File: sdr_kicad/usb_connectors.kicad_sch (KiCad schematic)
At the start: 10 parts, among them J1 USB_C_Receptacle, J2 USB_C_Receptacle, U10 USBLC6-2SC6, U11 USBLC6-2SC6

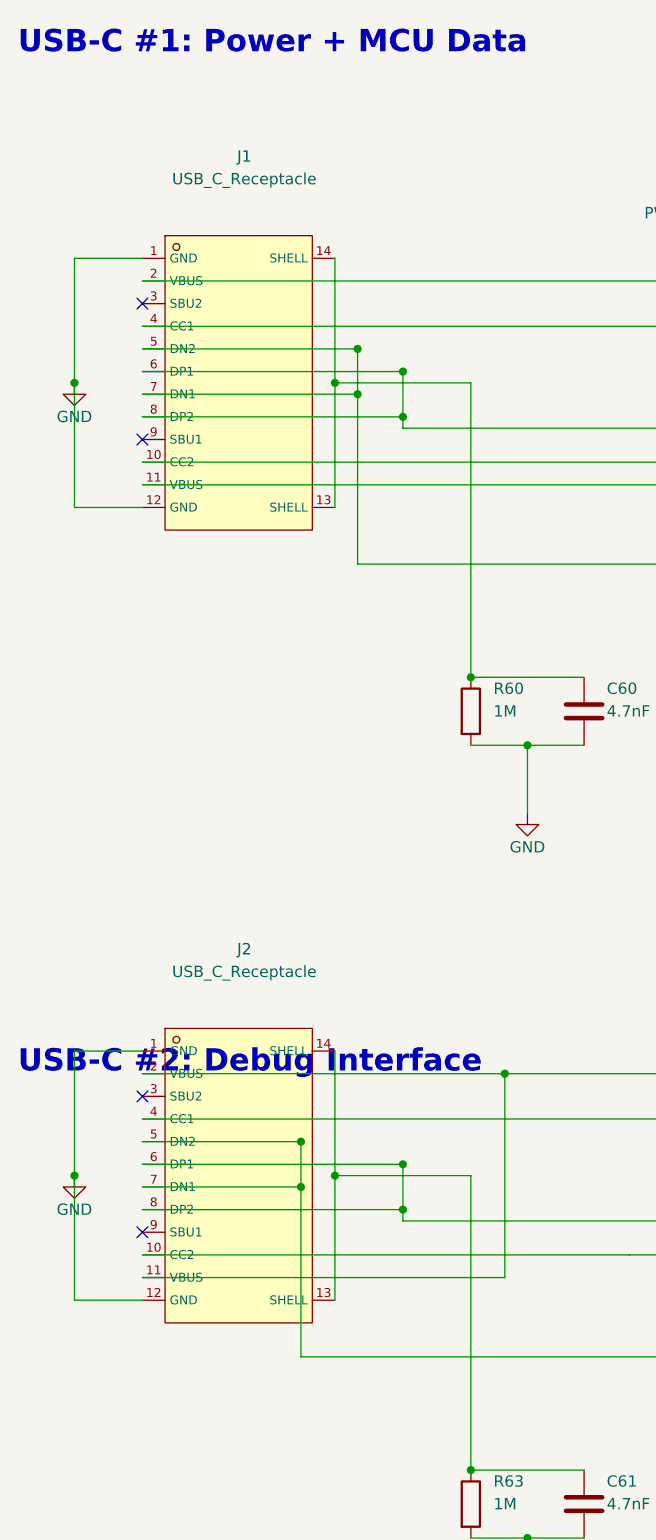
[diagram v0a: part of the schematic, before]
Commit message: add firmware and readme
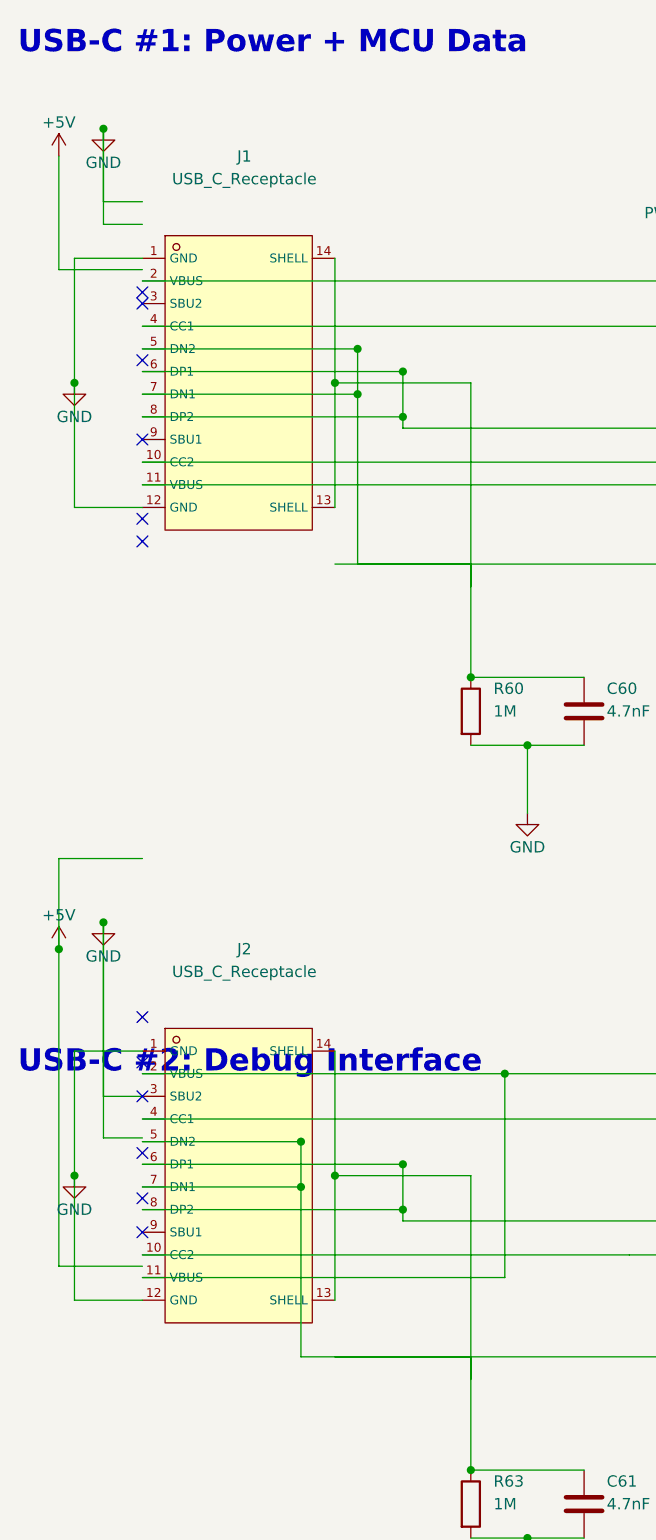
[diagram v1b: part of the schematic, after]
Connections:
- net GND: now also C61.1, J2.13 (SHELL), J2.14 (SHELL), J2.3 (SBU2), R63.1
- net at C60.1, J1.13 (SHELL), J1.14 (SHELL)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: now also J1.5 (DN2), J1.7 (DN1), U10.3 (I/O2)
- no-connect marks 4 -> 12
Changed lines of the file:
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@@
   (junction (at 76.2 96.52) (diameter 0) (color 0 0 0 0) (uuid "jct-rc1-top"))
   (junction (at 76.2 185.42) (diameter 0) (color 0 0 0 0) (uuid "jct-rc2-top"))
+  ; J1 missing connections
+  ; GND pins
+  (wire (pts (xy 39.37 45.72) (xy 35 45.72)) (uuid "wire-j1-gnd1-1"))
+  (wire (pts (xy 35 45.72) (xy 35 35)) (uuid "wire-j1-gnd1-2"))
+  (wire (pts (xy 39.37 43.18) (xy 35 43.18)) (uuid "wire-j1-gnd12-1"))
+  (wire (pts (xy 35 43.18) (xy 35 35)) (uuid "wire-j1-gnd12-2"))
+  (junction (at 35 35) (uuid "jct-j1-gnd"))
+  (symbol
+    (lib_id "power:GND")
+    (at 35 35 0)
+    (unit 1)
+    (exclude_from_sim no)
+    (in_bom no)
+    (on_board yes)
+    (dnp no)
+    (uuid "pwr-gnd-j1")
+    (property "Reference" "#PWR017"
+      (at 35 41.35 0)
+      (effects (font (size 1.27 1.27)) hide)
+    )
+    (property "Value" "GND"
+      (at 35 38.81 0)
+      (effects (font (size 1.27 1.27)))
+    )
+  )
+  ; VBUS pin 11
+  (wire (pts (xy 39.37 50.80) (xy 30 50.80)) (uuid "wire-j1-vbus11-1"))
+  (wire (pts (xy 30 50.80) (xy 30 38.1)) (uuid "wire-j1-vbus11-2"))
+  (symbol
+    (lib_id "power:+5V")
+    (at 30 38.1 0)
+    (unit 1)
+    (exclude_from_sim no)
+    (in_bom no)
+    (on_board yes)
+    (dnp no)
+    (uuid "pwr-5v-j1-vbus11")
+    (property "Reference" "#PWR018"
+      (at 30 41.91 0)
+      (effects (font (size 1.27 1.27)) hide)
+    )
+    (property "Value" "+5V"
+      (at 30 34.29 0)
+      (effects (font (size 1.27 1.27)))
+    )
+  )
+  ; SHELL pin 13
+  (wire (pts (xy 60.96 83.82) (xy 76.2 83.82)) (uuid "wire-j1-shell13-1"))
+  (wire (pts (xy 76.2 83.82) (xy 76.2 86.36)) (uuid "wire-j1-shell13-2"))
+  ; No-connect flags for J1
+  (no_connect (at 39.37 53.34) (uuid "nc-j1-sbu2"))
+  (no_connect (at 39.37 60.96) (uuid "nc-j1-dn2"))
+  (no_connect (at 39.37 78.74) (uuid "nc-j1-dp2"))
+  (no_connect (at 39.37 81.28) (uuid "nc-j1-sbu1"))
+  ; J2 missing connections
+  ; GND pins
+  (wire (pts (xy 39.37 143.51) (xy 35 143.51)) (uuid "wire-j2-gnd1-1"))
+  (wire (pts (xy 35 143.51) (xy 35 124)) (uuid "wire-j2-gnd1-2"))
+  (wire (pts (xy 39.37 148.17) (xy 35 148.17)) (uuid "wire-j2-gnd12-1"))
+  (wire (pts (xy 35 148.17) (xy 35 124)) (uuid "wire-j2-gnd12-2"))
+  (junction (at 35 124) (uuid "jct-j2-gnd"))
+  (symbol
+    (lib_id "power:GND")
+    (at 35 124 0)
+    (unit 1)
+    (exclude_from_sim no)
+    (in_bom no)
+    (on_board yes)
+    (dnp no)
+    (uuid "pwr-gnd-j2")
+    (property "Reference" "#PWR019"
+      (at 35 130.35 0)
+      (effects (font (size 1.27 1.27)) hide)
+    )
+    (property "Value" "GND"
+      (at 35 127.81 0)
+      (effects (font (size 1.27 1.27)))
+    )
+  )
+  ; VBUS pins 2 and 11
+  (wire (pts (xy 39.37 116.84) (xy 30 116.84)) (uuid "wire-j2-vbus2-1"))
+  (wire (pts (xy 30 116.84) (xy 30 127)) (uuid "wire-j2-vbus2-2"))
+  (wire (pts (xy 39.37 162.56) (xy 30 162.56)) (uuid "wire-j2-vbus11-1"))
+  (wire (pts (xy 30 162.56) (xy 30 127)) (uuid "wire-j2-vbus11-2"))
+  (junction (at 30 127) (uuid "jct-j2-vbus"))
+  (symbol
+    (lib_id "power:+5V")
+    (at 30 127 0)
+    (unit 1)
+    (exclude_from_sim no)
+    (in_bom no)
+    (on_board yes)
+    (dnp no)
+    (uuid "pwr-5v-j2-vbus")
+    (property "Reference" "#PWR020"
+      (at 30 130.81 0)
+      (effects (font (size 1.27 1.27)) hide)
+    )
+    (property "Value" "+5V"
+      (at 30 123.19 0)
+      (effects (font (size 1.27 1.27)))
+    )
+  )
+  ; SHELL pin 13
+  (wire (pts (xy 60.96 172.72) (xy 76.2 172.72)) (uuid "wire-j2-shell13-1"))
+  (wire (pts (xy 76.2 172.72) (xy 76.2 175.26)) (uuid "wire-j2-shell13-2"))
+  ; No-connect flags for J2
+  (no_connect (at 39.37 134.62) (uuid "nc-j2-sbu2"))
+  (no_connect (at 39.37 139.7) (uuid "nc-j2-dn2"))
+  (no_connect (at 39.37 149.86) (uuid "nc-j2-dp2"))
+  (no_connect (at 39.37 154.94) (uuid "nc-j2-sbu1"))
 )
